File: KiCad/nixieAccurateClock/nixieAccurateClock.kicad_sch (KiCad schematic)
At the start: 8 parts, among them J1 Conn_01x02_Pin, J2 Conn_01x02_Pin, J3 Conn_01x02_Pin, SW1 SW_DIP_x08

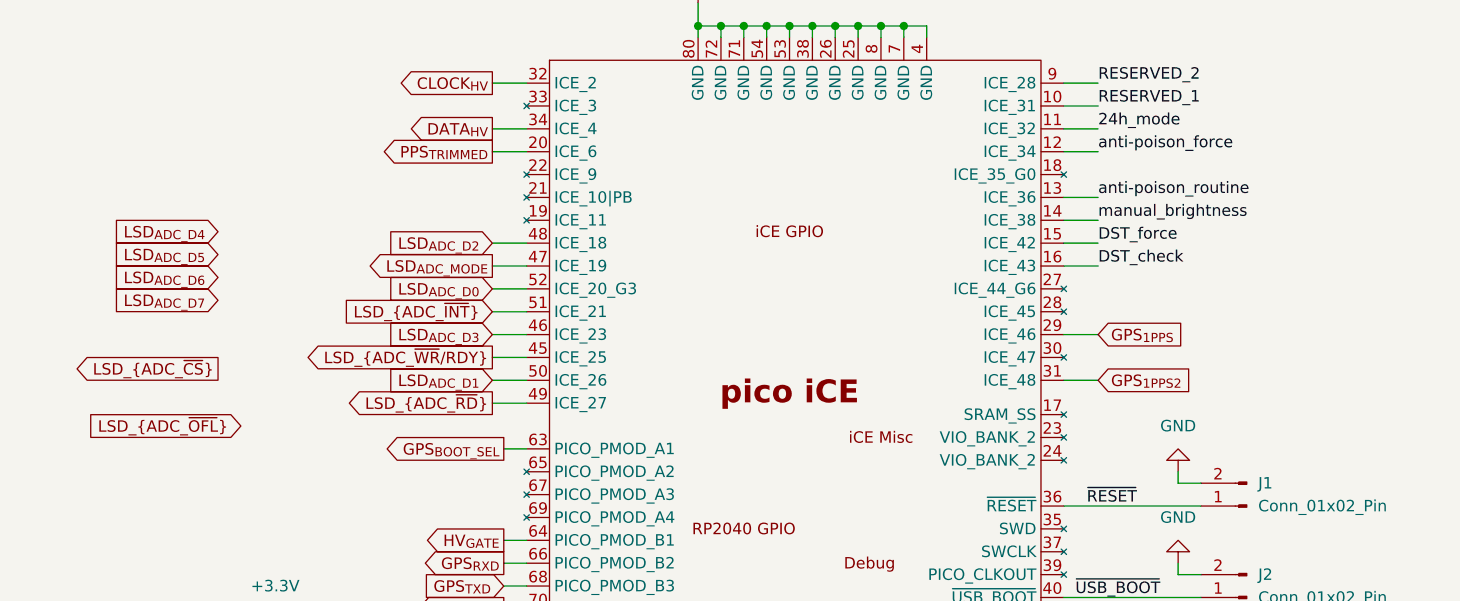
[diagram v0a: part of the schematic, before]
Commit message: ERC and DRC pass
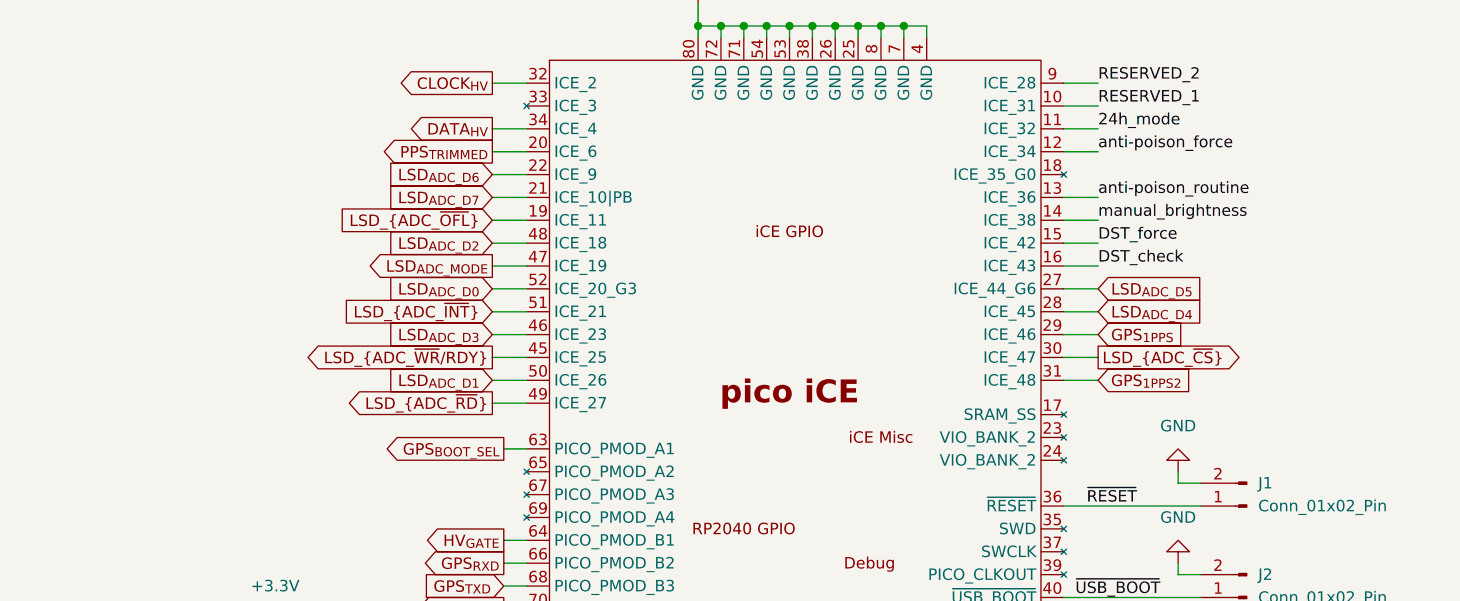
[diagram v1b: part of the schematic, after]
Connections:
- net LSD_{ADC_D4}: now also U1.28 (ICE_45)
- net LSD_{ADC_D5}: now also U1.27 (ICE_44_G6)
- net LSD_{ADC_D6}: now also U1.22 (ICE_9)
- net LSD_{ADC_D7}: now also U1.21 (ICE_10|PB)
- net LSD_{ADC_~{CS}}: now also U1.30 (ICE_47)
- net LSD_{ADC_~{OFL}}: now also U1.19 (ICE_11)
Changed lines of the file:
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@@
+    (stroke (width 0) (type default))
+  )
+  (wire (pts (xy 134.62 53.34) (xy 138.43 53.34))
     (stroke (width 0) (type default))
   )
@@
     (stroke (width 0) (type default))
   )
+  (wire (pts (xy 134.62 58.42) (xy 138.43 58.42))
+    (stroke (width 0) (type default))
+  )
   (wire (pts (xy 71.12 35.56) (xy 74.93 35.56))
     (stroke (width 0) (type default))
@@
     (stroke (width 0) (type default))
   )
+  (wire (pts (xy 71.12 40.64) (xy 74.93 40.64))
+    (stroke (width 0) (type default))
+  )
   (wire (pts (xy 93.98 21.59) (xy 93.98 22.86))
     (stroke (width 0) (type default))
   )
+  (wire (pts (xy 134.62 50.8) (xy 138.43 50.8))
+    (stroke (width 0) (type default))
+  )
   (wire (pts (xy 46.99 99.06) (xy 46.99 97.79))
     (stroke (width 0) (type default))
@@
     (stroke (width 0) (type default))
   )
+  (wire (pts (xy 71.12 43.18) (xy 74.93 43.18))
+    (stroke (width 0) (type default))
+  )
   (wire (pts (xy 242.57 83.82) (xy 246.38 83.82))
     (stroke (width 0) (type default))
@@
   )
   (wire (pts (xy 134.62 43.18) (xy 138.43 43.18))
+    (stroke (width 0) (type default))
+  )
+  (wire (pts (xy 71.12 38.1) (xy 74.93 38.1))
     (stroke (width 0) (type default))
   )
@@
     )
   )
-  (global_label "LSD_{ADC_D4}" (shape input) (at 40.64 44.45 180) (fields_autoplaced)
-    (effects (font (size 1.27 1.27)) (justify right))
-    (property "Intersheetrefs" "${INTERSHEET_REFS}" (at 28.4358 44.45 0)
-      (effects (font (size 1.27 1.27)) (justify right) hide)
+  (global_label "LSD_{ADC_D4}" (shape input) (at 138.43 53.34 0) (fields_autoplaced)
+    (effects (font (size 1.27 1.27)) (justify left))
+    (property "Intersheetrefs" "${INTERSHEET_REFS}" (at 150.6342 53.34 0)
+      (effects (font (size 1.27 1.27)) (justify left) hide)
     )
   )
@@
     )
   )
-  (global_label "LSD_{ADC_D7}" (shape input) (at 40.64 52.07 180) (fields_autoplaced)
-    (effects (font (size 1.27 1.27)) (justify right))
-    (property "Intersheetrefs" "${INTERSHEET_REFS}" (at 28.4358 52.07 0)
-      (effects (font (size 1.27 1.27)) (justify right) hide)
-    )
-  )
-  (global_label "LSD_{ADC_D6}" (shape input) (at 40.64 49.53 180) (fields_autoplaced)
-    (effects (font (size 1.27 1.27)) (justify right))
-    (property "Intersheetrefs" "${INTERSHEET_REFS}" (at 28.4358 49.53 0)
+  (global_label "LSD_{ADC_D7}" (shape input) (at 71.12 40.64 180) (fields_autoplaced)
+    (effects (font (size 1.27 1.27)) (justify right))
+    (property "Intersheetrefs" "${INTERSHEET_REFS}" (at 58.9158 40.64 0)
+      (effects (font (size 1.27 1.27)) (justify right) hide)
+    )
+  )
+  (global_label "LSD_{ADC_D6}" (shape input) (at 71.12 38.1 180) (fields_autoplaced)
+    (effects (font (size 1.27 1.27)) (justify right))
+    (property "Intersheetrefs" "${INTERSHEET_REFS}" (at 58.9158 38.1 0)
       (effects (font (size 1.27 1.27)) (justify right) hide)
     )
@@
     )
   )
-  (global_label "LSD_{ADC_~{OFL}}" (shape input) (at 43.18 66.04 180) (fields_autoplaced)
-    (effects (font (size 1.27 1.27)) (justify right))
-    (property "Intersheetrefs" "${INTERSHEET_REFS}" (at 30.2016 66.04 0)
-      (effects (font (size 1.27 1.27)) (justify right) hide)
-    )
-  )
-  (global_label "LSD_{ADC_~{CS}}" (shape output) (at 40.64 59.69 180) (fields_autoplaced)
-    (effects (font (size 1.27 1.27)) (justify right))
-    (property "Intersheetrefs" "${INTERSHEET_REFS}" (at 28.4358 59.69 0)
-      (effects (font (size 1.27 1.27)) (justify right) hide)
+  (global_label "LSD_{ADC_~{OFL}}" (shape input) (at 71.12 43.18 180) (fields_autoplaced)
+    (effects (font (size 1.27 1.27)) (justify right))
+    (property "Intersheetrefs" "${INTERSHEET_REFS}" (at 58.1416 43.18 0)
+      (effects (font (size 1.27 1.27)) (justify right) hide)
+    )
+  )
+  (global_label "LSD_{ADC_~{CS}}" (shape output) (at 138.43 58.42 0) (fields_autoplaced)
+    (effects (font (size 1.27 1.27)) (justify left))
+    (property "Intersheetrefs" "${INTERSHEET_REFS}" (at 150.6342 58.42 0)
+      (effects (font (size 1.27 1.27)) (justify left) hide)
     )
   )
@@
     )
   )
-  (global_label "LSD_{ADC_D5}" (shape input) (at 40.64 46.99 180) (fields_autoplaced)
-    (effects (font (size 1.27 1.27)) (justify right))
-    (property "Intersheetrefs" "${INTERSHEET_REFS}" (at 28.4358 46.99 0)
-      (effects (font (size 1.27 1.27)) (justify right) hide)
-    )
-  )
+  (global_label "LSD_{ADC_D5}" (shape input) (at 138.43 50.8 0) (fields_autoplaced)
+    (effects (font (size 1.27 1.27)) (justify left))
+    (property "Intersheetrefs" "${INTERSHEET_REFS}" (at 150.6342 50.8 0)
+      (effects (font (size 1.27 1.27)) (justify left) hide)
+    )
+  )
